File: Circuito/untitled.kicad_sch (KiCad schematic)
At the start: 1 part, among them U1 ESP32-S3-WROOM-1

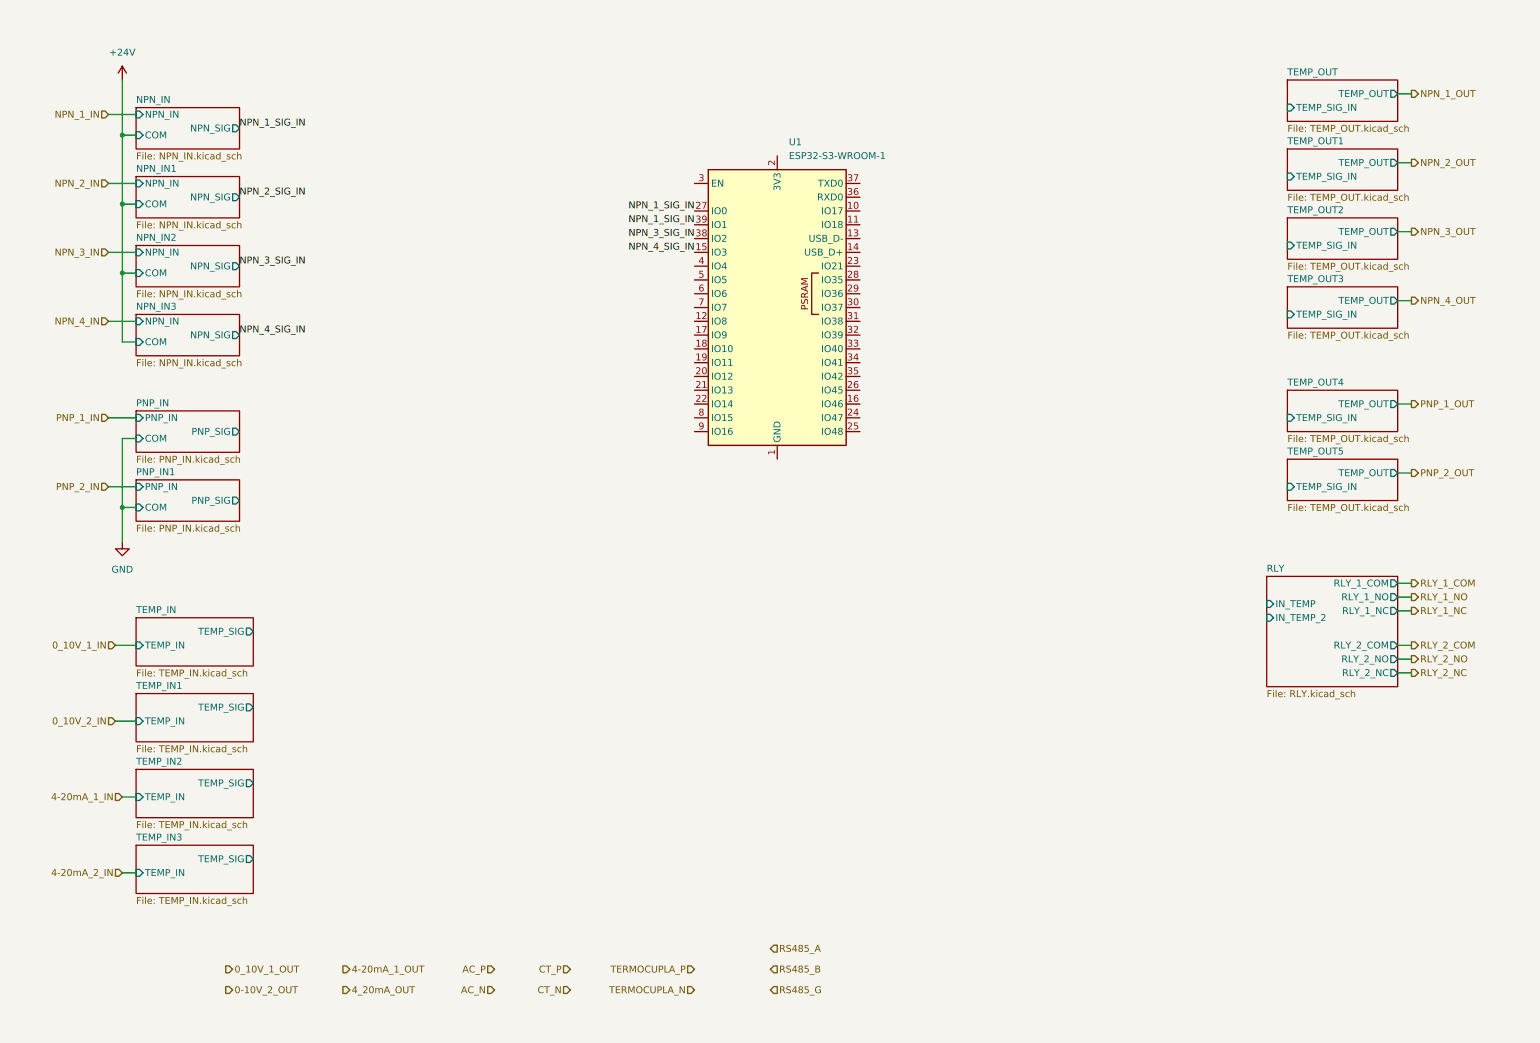
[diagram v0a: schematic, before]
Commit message: commit
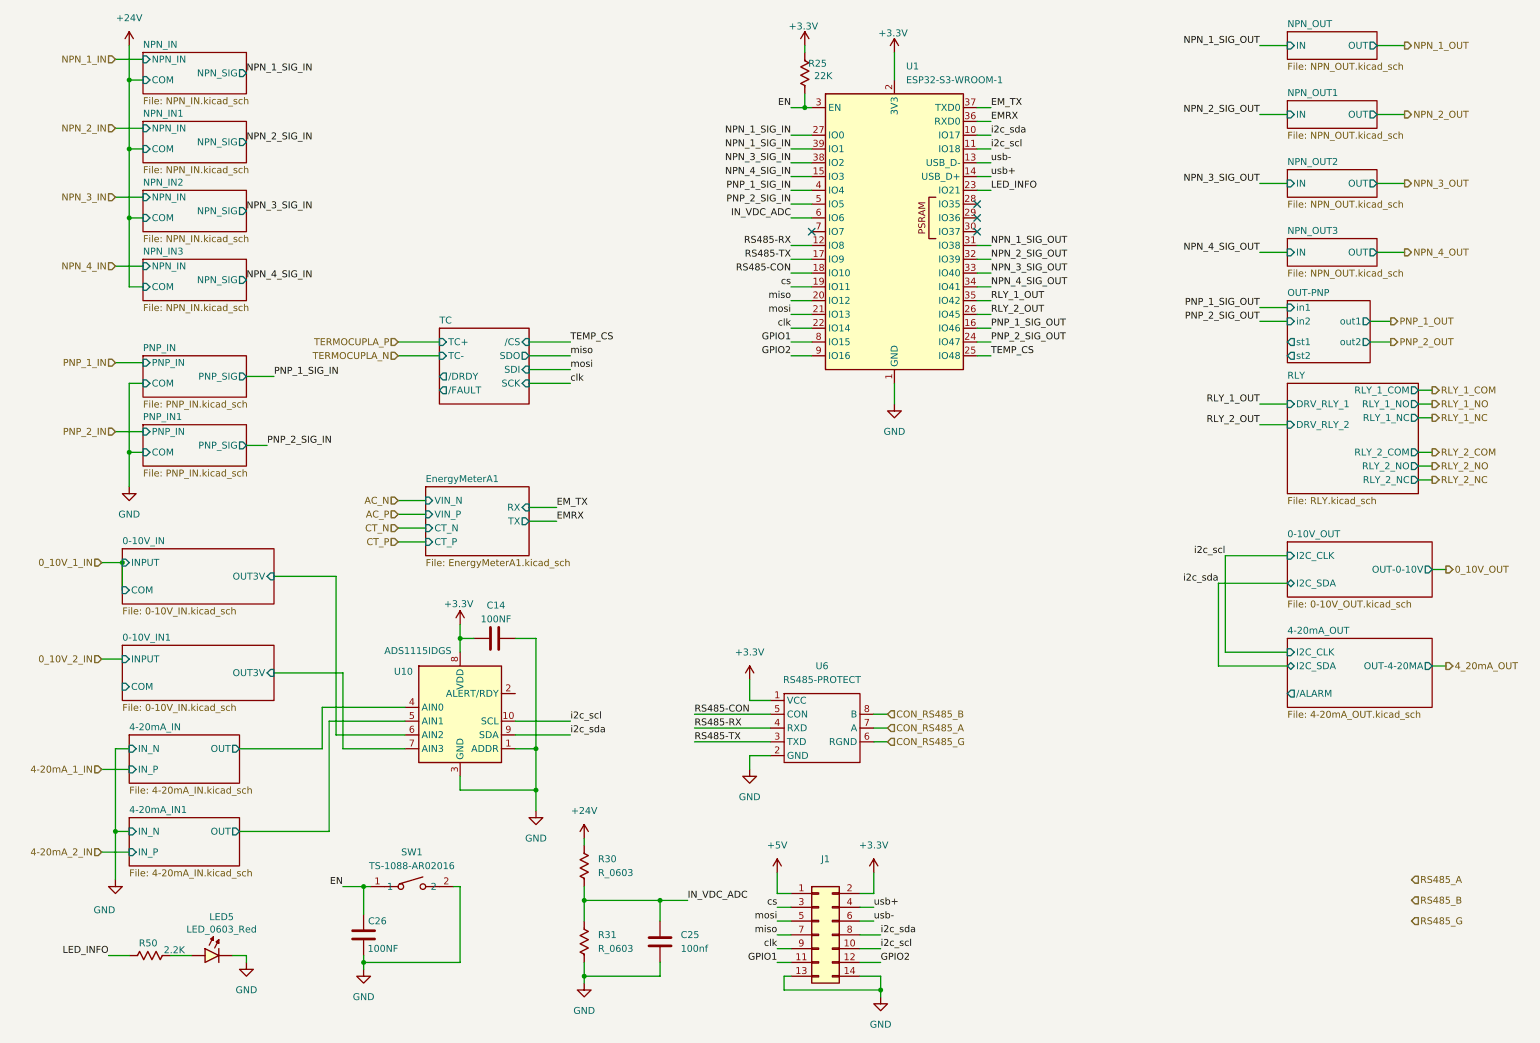
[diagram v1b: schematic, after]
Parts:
- added C14, C26: 100NF, PCM_Capacitor_SMD_AKL:C_0603_1608Metric, symbol Capacitor_AKL:C_0603
- added C25: 100nf, PCM_Capacitor_SMD_AKL:C_0603_1608Metric, symbol Capacitor_AKL:C_0603
- added J1: Conn_02x07_Odd_Even, Connector_PinHeader_2.54mm:PinHeader_2x07_P2.54mm_Vertical, symbol Connector_Generic:Conn_02x07_Odd_Even
- added LED5: LED_0603_Red, PCM_Resistor_SMD_AKL:R_0603_1608Metric, symbol LED_AKL:LED_0603_Red
- added R25: 22K, PCM_Resistor_SMD_AKL:R_0603_1608Metric, symbol Resistor_US_AKL:R_0603
- added R30, R31: R_0603, PCM_Resistor_SMD_AKL:R_0603_1608Metric, symbol Resistor_US_AKL:R_0603
- added R50: 2.2K, PCM_Resistor_SMD_AKL:R_0603_1608Metric, symbol Resistor_US_AKL:R_0603
- added SW1: TS-1088-AR02016, EasyEDA:SW-SMD_L3.9-W3.0-P4.45, symbol EasyEDA:TS-1088-AR02016
- added U10: ADS1115IDGS, Package_SO:TSSOP-10_3x3mm_P0.5mm, symbol Analog_ADC:ADS1115IDGS
- added U6: RS485-PROTECT, MG_footprints:RS-485-PROTECT, symbol MG_CONNECTORS:RS485-PROTECT
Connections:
- net +24V: now also R30.1
- net GND: now also U1.1 (GND), U1.40 (GND), U1.41 (GND), C14.2, C25.2, C26.1, J1.13 (Pin_13), J1.14 (Pin_14), LED5.1 (K), R31.2, SW1.2, U10.1 (ADDR), U10.3 (GND), U6.2 (GND)
- net i2c_sda: now reaches U1.10 (IO17)
- net i2c_sda: now also J1.8 (Pin_8), U10.9 (SDA)
- net i2c_scl: now reaches U1.11 (IO18)
- net i2c_scl: now also J1.10 (Pin_10), U10.10 (SCL)
- net RS485-RX: now reaches U1.12 (IO8)
- net RS485-RX: now also U6.4 (RXD)
- net usb-: now reaches U1.13 (USB_D-)
- net usb-: now also J1.6 (Pin_6)
- net usb+: now reaches U1.14 (USB_D+)
- net usb+: now also J1.4 (Pin_4)
- net PNP_1_SIG_OUT: now reaches U1.16 (IO46)
- net RS485-TX: now reaches U1.17 (IO9)
- net RS485-TX: now also U6.3 (TXD)
- net RS485-CON: now reaches U1.18 (IO10)
- net RS485-CON: now also U6.5 (CON)
- net cs: now reaches U1.19 (IO11)
- net cs: now also J1.3 (Pin_3)
- net +3.3V: now reaches U1.2 (3V3)
- net +3.3V: now also C14.1, J1.2 (Pin_2), R25.2, U10.8 (VDD), U6.1 (VCC)
- net miso: now reaches U1.20 (IO12)
- net miso: now also J1.7 (Pin_7)
- net mosi: now reaches U1.21 (IO13)
- net mosi: now also J1.5 (Pin_5)
- net clk: now reaches U1.22 (IO14)
- net clk: now also J1.9 (Pin_9)
- net LED_INFO: now reaches U1.23 (IO21)
- net LED_INFO: now also R50.2
- net PNP_2_SIG_OUT: now reaches U1.24 (IO47)
- net TEMP_CS: now reaches U1.25 (IO48)
- net RLY_2_OUT: now reaches U1.26 (IO45)
- net EN: now reaches U1.3 (EN)
- net EN: now also C26.2, R25.1, SW1.1
- net NPN_1_SIG_OUT: now reaches U1.31 (IO38)
- net NPN_2_SIG_OUT: now reaches U1.32 (IO39)
- net NPN_3_SIG_OUT: now reaches U1.33 (IO40)
- net NPN_4_SIG_OUT: now reaches U1.34 (IO41)
- net RLY_1_OUT: now reaches U1.35 (IO42)
- net EMRX: now reaches U1.36 (RXD0)
- net EM_TX: now reaches U1.37 (TXD0)
- net PNP_1_SIG_IN: now reaches U1.4 (IO4)
- net PNP_2_SIG_IN: now reaches U1.5 (IO5)
- net IN_VDC_ADC: now reaches U1.6 (IO6)
- net IN_VDC_ADC: now also C25.1, R30.2, R31.1
- net GPIO1: now reaches U1.8 (IO15)
- net GPIO1: now also J1.11 (Pin_11)
- net GPIO2: now reaches U1.9 (IO16)
- net GPIO2: now also J1.12 (Pin_12)
- new net: LED5.2 (A), R50.1
- new net +5V: J1.1 (Pin_1)
- new net 0-10V_IN/OUT3V: U10.6 (AIN2)
- new net 0-10V_IN1/OUT3V: U10.7 (AIN3)
- new net 4-20mA_IN/OUT: U10.4 (AIN0)
- new net 4-20mA_IN1/OUT: U10.5 (AIN1)
- new net CON_RS485_A: U6.7 (A)
- new net CON_RS485_B: U6.8 (B)
- new net CON_RS485_G: U6.6 (RGND)
- no-connect marks 0 -> 4
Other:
- removed sheet TEMP_IN
- removed sheet TEMP_IN1
- removed sheet TEMP_IN2
- removed sheet TEMP_IN3
- removed sheet TEMP_OUT
- removed sheet TEMP_OUT1
- removed sheet TEMP_OUT2
- removed sheet TEMP_OUT3
- removed sheet TEMP_OUT4
- removed sheet TEMP_OUT5
- added sheet 0-10V_IN (0-10V_IN.kicad_sch)
- added sheet 0-10V_IN1 (0-10V_IN.kicad_sch)
- added sheet 0-10V_OUT (0-10V_OUT.kicad_sch)
- added sheet 4-20mA_IN (4-20mA_IN.kicad_sch)
- added sheet 4-20mA_IN1 (4-20mA_IN.kicad_sch)
- added sheet 4-20mA_OUT (4-20mA_OUT.kicad_sch)
- added sheet EnergyMeterA1 (EnergyMeterA1.kicad_sch)
- added sheet NPN_OUT (NPN_OUT.kicad_sch)
- added sheet NPN_OUT1 (NPN_OUT.kicad_sch)
- added sheet NPN_OUT2 (NPN_OUT.kicad_sch)
- added sheet NPN_OUT3 (NPN_OUT.kicad_sch)
- added sheet OUT-PNP (OUT-PNP.kicad_sch)
- added sheet TC (TC.kicad_sch)
- sheet RLY ports: added DRV_RLY_1, DRV_RLY_2; removed IN_TEMP, IN_TEMP_2
- moved on the sheet: U1

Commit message: Last commit
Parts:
- U6: footprint MG_footprints:RS-485-PROTECT -> Package_SO:SOIC-8_5.3x6.2mm_P1.27mm
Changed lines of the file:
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@@
 			)
 		)
-		(property "Footprint" "MG_footprints:RS-485-PROTECT"
+		(property "Footprint" "Package_SO:SOIC-8_5.3x6.2mm_P1.27mm"
 			(at 152.4 143.51 0)
 			(effects
